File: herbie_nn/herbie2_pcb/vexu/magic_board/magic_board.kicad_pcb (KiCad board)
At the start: 2 copper layers, 66 x 47.5 mm, 53 parts, among them J1 4P4C, J2 Conn_ARM_JTAG_SWD_10, J3 USB_C_Receptacle_USB2.0_14P, J4 Micro_SD_Card, U2 AT25SF081-SSHD-X, U3 BD33FC0WEFJ, U4 ATSAMD51J19A-A, U5 LS7366R, U6 LS7366R, U7 LS7366R, U8 LS7366R, Y1 32.768KHz

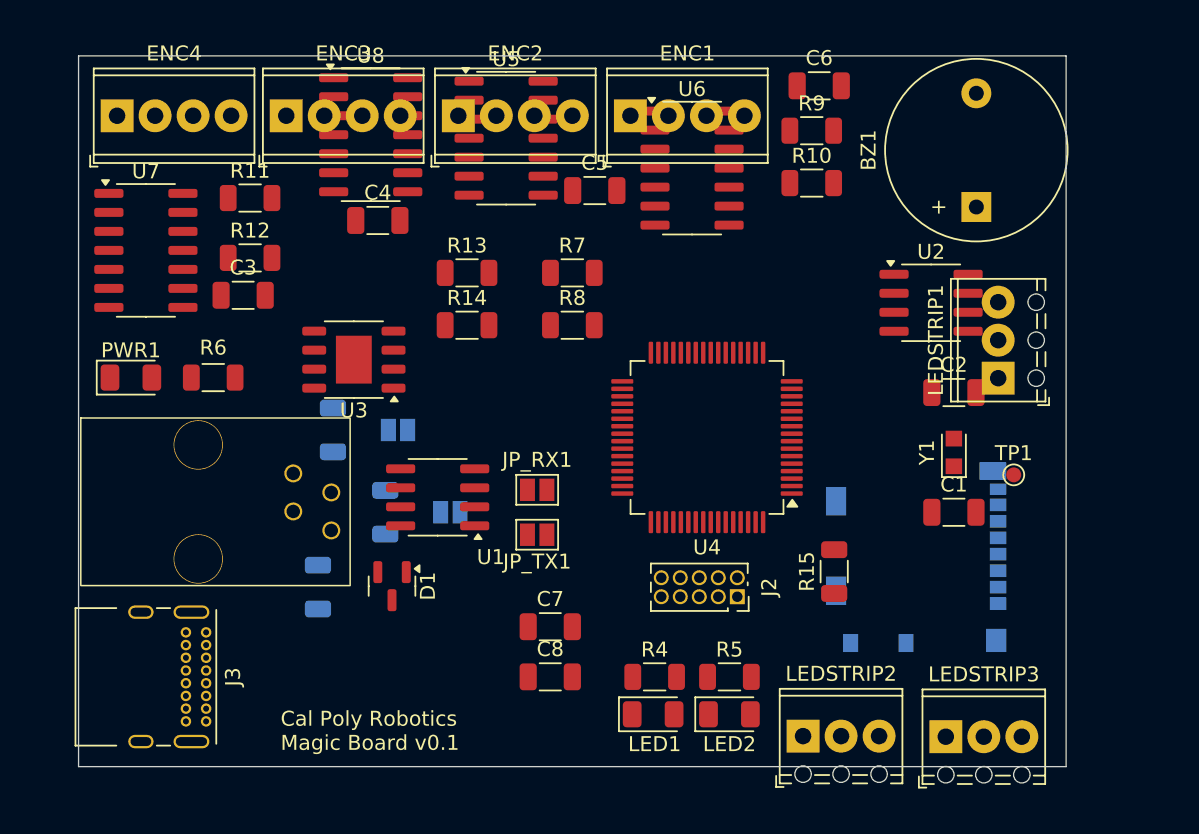
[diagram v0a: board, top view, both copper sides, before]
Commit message: updated board
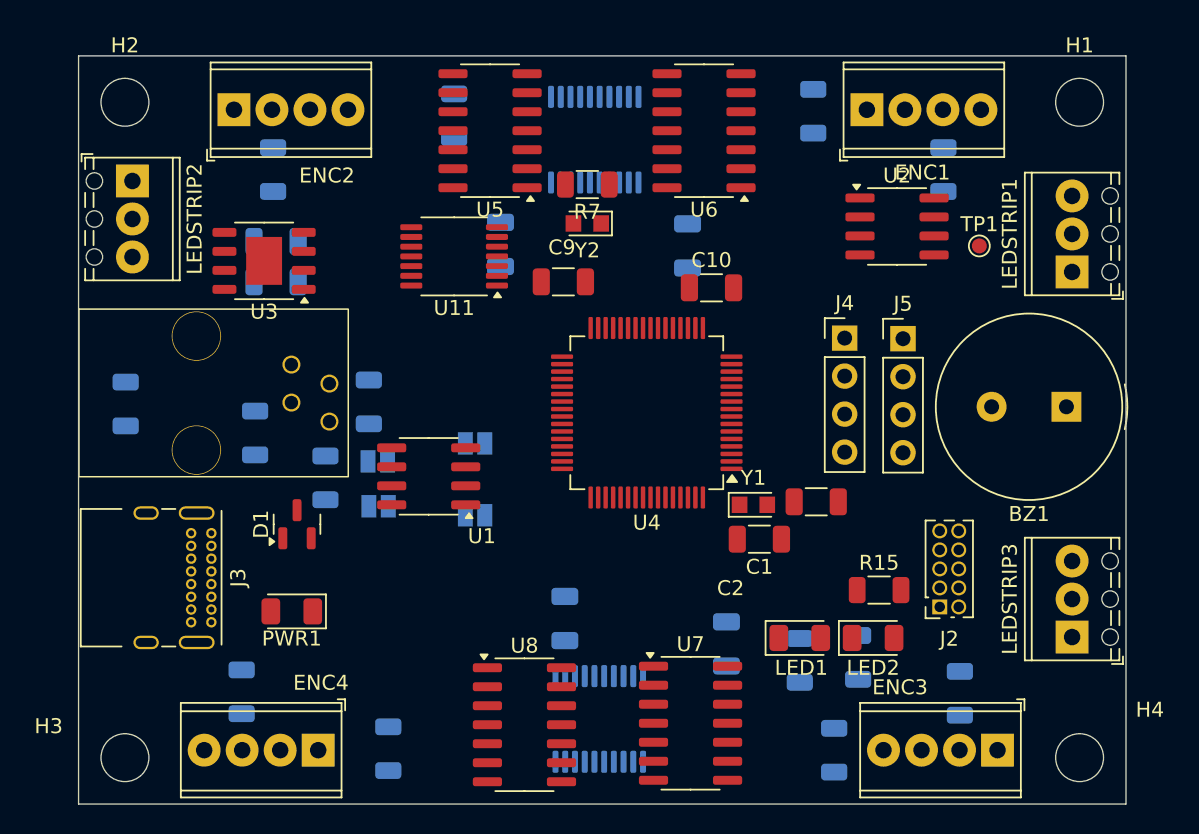
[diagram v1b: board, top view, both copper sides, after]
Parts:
- removed R8: R, Resistor_SMD:R_1206_3216Metric
- added C10: C, Capacitor_SMD:C_1206_3216Metric, F.Cu at (67.8, 77.5)
- added C9: C, Capacitor_SMD:C_1206_3216Metric, F.Cu at (57.9, 77.1)
- added H1: MountingHole, MountingHole:MountingHole_3.2mm_M3_DIN965, F.Cu at (92.4, 65.1)
- added H2: MountingHole, MountingHole:MountingHole_3.2mm_M3_DIN965, F.Cu at (28.6, 65.1)
- added H3: MountingHole, MountingHole:MountingHole_3.2mm_M3_DIN965, F.Cu at (28.6, 108.9)
- added H4: MountingHole, MountingHole:MountingHole_3.2mm_M3_DIN965, F.Cu at (92.4, 108.9)
- added J5: Conn_01x04_Pin, Connector_PinHeader_2.54mm:PinHeader_1x04_P2.54mm_Vertical, F.Cu at (80.6, 80.9)
- added R16: R, Resistor_SMD:R_1206_3216Metric, B.Cu at (46.2, 108.3)
- added R17: R, Resistor_SMD:R_1206_3216Metric, B.Cu at (36.4, 104.5)
- added U10: SN74LVC245APW, Package_SO:TSSOP-20_4.4x6.5mm_P0.65mm, B.Cu at (60.3, 106.3)
- added U11: 74HC14, Package_SO:TSSOP-14_4.4x5mm_P0.65mm, F.Cu at (50.6, 75.4)
- added U9: SN74LVC245APW, Package_SO:TSSOP-20_4.4x6.5mm_P0.65mm, B.Cu at (60.0, 67.6)
- added Y2: 20MHz, Crystal:Crystal_SMD_2012-2Pin_2.0x1.2mm_HandSoldering, F.Cu at (59.5, 73.2)
- BZ1: footprint Buzzer_Beeper:Buzzer_12x9.5RM7.6 -> Buzzer_Beeper:Buzzer_TDK_PS1240P02BT_D12.2mm_H6.5mm
- C3, C4, C5, C6, C7, C8, JP_RX1, JP_TX1, R10, R11, R12, R13, R14, R4, R5, R6, R9: moved to B.Cu
- J4: value Micro_SD_Card -> Conn_01x04_Pin; footprint Connector_Card:microSD_HC_Molex_104031-0811 -> Connector_PinHeader_2.54mm:PinHeader_1x04_P2.54mm_Vertical; moved to F.Cu
- R7: value R -> 1M
- moved ENC3 63.7 mm to (86.9, 108.4), turned to 180 degrees
- moved LEDSTRIP2 58.2 mm to (29.1, 70.4), turned to -90 degrees
- moved U7 48.2 mm to (66.4, 106.6)
- moved ENC4 44.5 mm to (41.5, 108.4), turned to 180 degrees
- moved R13 43.3 mm to (84.4, 104.6), turned to 90 degrees
- moved U8 40.7 mm to (55.3, 106.7)
- moved C6 39.5 mm to (58.0, 99.6), turned to 90 degrees
- moved R14 37.5 mm to (76.0, 108.4), turned to 90 degrees
- moved C8 32.1 mm to (38.7, 77.1), turned to 180 degrees
- moved C7 31.6 mm to (38.7, 74.4), turned to 180 degrees
- moved C5 31.6 mm to (68.8, 101.3), turned to -90 degrees
- moved C4 20.8 mm to (66.2, 74.7), turned to -90 degrees
- moved PWR1 19.0 mm to (39.8, 99.1), turned to 180 degrees
- moved C3 17.5 mm to (53.7, 74.6), turned to -90 degrees
- moved R12 16.6 mm to (50.6, 66.0), turned to -90 degrees
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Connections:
- BZ1 pad 1: unconnected-(BZ1-+-Pad1) -> /BUZ_PIN
- ENC1 pad 2: unconnected-(ENC1-Pin_2-Pad2) -> /A1_IN
- ENC1 pad 3: unconnected-(ENC1-Pin_3-Pad3) -> /B1_IN
- ENC2 pad 2: unconnected-(ENC2-Pin_2-Pad2) -> /A2_IN
- ENC2 pad 3: unconnected-(ENC2-Pin_3-Pad3) -> /B2_IN
- ENC3 pad 2: unconnected-(ENC3-Pin_2-Pad2) -> /A3_IN
- ENC3 pad 3: unconnected-(ENC3-Pin_3-Pad3) -> /B3_IN
- ENC4 pad 2: unconnected-(ENC4-Pin_2-Pad2) -> /A4_IN
- ENC4 pad 3: unconnected-(ENC4-Pin_3-Pad3) -> /B4_IN
- LEDSTRIP1 pad 1: unconnected-(LEDSTRIP1-Pin_1-Pad1) -> GND
- LEDSTRIP1 pad 2: unconnected-(LEDSTRIP1-Pin_2-Pad2) -> /LED_SIG1
- LEDSTRIP1 pad 3: unconnected-(LEDSTRIP1-Pin_3-Pad3) -> +12V
- LEDSTRIP2 pad 1: unconnected-(LEDSTRIP2-Pin_1-Pad1) -> GND
- LEDSTRIP2 pad 2: unconnected-(LEDSTRIP2-Pin_2-Pad2) -> /LED_SIG2
- LEDSTRIP2 pad 3: unconnected-(LEDSTRIP2-Pin_3-Pad3) -> +12V
- LEDSTRIP3 pad 1: unconnected-(LEDSTRIP3-Pin_1-Pad1) -> GND
- LEDSTRIP3 pad 2: unconnected-(LEDSTRIP3-Pin_2-Pad2) -> /LED_SIG3
- LEDSTRIP3 pad 3: unconnected-(LEDSTRIP3-Pin_3-Pad3) -> +12V
- R10 pad 1: Net-(U6-b) -> /B1_IN
- R10 pad 2: unconnected-(R10-Pad2) -> Net-(U9-A2)
- R11 pad 1: Net-(U7-a) -> /A2_IN
- R11 pad 2: unconnected-(R11-Pad2) -> Net-(U9-A3)
- R12 pad 1: Net-(U7-b) -> /B2_IN
- R12 pad 2: unconnected-(R12-Pad2) -> Net-(U9-A4)
- R13 pad 1: Net-(U8-a) -> /A3_IN
- R13 pad 2: unconnected-(R13-Pad2) -> Net-(U10-A5)
- R14 pad 1: Net-(U8-b) -> /B3_IN
- R14 pad 2: unconnected-(R14-Pad2) -> Net-(U10-A6)
- R7 pad 1: Net-(U5-a) -> Net-(U5-fcki)
- R7 pad 2: unconnected-(R7-Pad2) -> /EN_CLK
- R9 pad 1: Net-(U6-a) -> /A1_IN
- R9 pad 2: unconnected-(R9-Pad2) -> Net-(U9-A1)
- U4 pad 10: unconnected-(U4-PB07-Pad10) -> /ENC4_SS
- U4 pad 11: unconnected-(U4-PB08-Pad11) -> /BUZ_PIN
- U4 pad 13: unconnected-(U4-PA04-Pad13) -> /SERCOM0.0
- U4 pad 14: unconnected-(U4-PA05-Pad14) -> /SERCOM0.1
- U4 pad 15: unconnected-(U4-PA06-Pad15) -> /SERCOM0.2
- U4 pad 16: unconnected-(U4-PA07-Pad16) -> /SERCOM0.3
- U4 pad 3: unconnected-(U4-PA02-Pad3) -> /DAC_OUT0
- U4 pad 35: unconnected-(U4-PA16-Pad35) -> /SERCOM1.0
- U4 pad 36: unconnected-(U4-PA17-Pad36) -> /SERCOM1.1
- U4 pad 37: unconnected-(U4-PA18-Pad37) -> /SERCOM1.2
- U4 pad 38: unconnected-(U4-PA19-Pad38) -> /SERCOM1.3
- U4 pad 5: unconnected-(U4-PB04-Pad5) -> /ENC1_SS
- U4 pad 6: unconnected-(U4-PB05-Pad6) -> /ENC2_SS
- U4 pad 62: unconnected-(U4-PB01-Pad62) -> /LED_SIG3
- U4 pad 63: unconnected-(U4-PB02-Pad63) -> /LED_SIG2
- U4 pad 64: unconnected-(U4-PB03-Pad64) -> /LED_SIG1
- U4 pad 9: unconnected-(U4-PB06-Pad9) -> /ENC3_SS
- U5 pad 1: unconnected-(U5-fcko-Pad1) -> /EN_CLK
- U5 pad 11: Net-(U5-b) -> /B1
- U5 pad 12: Net-(U5-a) -> /A1
- U5 pad 2: unconnected-(U5-fcki-Pad2) -> Net-(U5-fcki)
- U6 pad 11: Net-(U6-b) -> /B2
- U6 pad 12: Net-(U6-a) -> /A2
- U6 pad 2: unconnected-(U6-fcki-Pad2) -> /OUT_CLK
- U7 pad 11: Net-(U7-b) -> /B3
- U7 pad 12: Net-(U7-a) -> /A3
- U7 pad 2: unconnected-(U7-fcki-Pad2) -> /OUT_CLK
- U8 pad 11: Net-(U8-b) -> /B4
- U8 pad 12: Net-(U8-a) -> /A4
- U8 pad 2: unconnected-(U8-fcki-Pad2) -> /OUT_CLK
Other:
- board size 66 x 47.5 mm -> 70 x 50 mm
- board text removed: "Cal Poly Robotics Magic Board v0.1"
